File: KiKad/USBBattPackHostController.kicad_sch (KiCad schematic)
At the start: 21 parts, among them SW301 Reset, U305 MIC5201-3.3YS, U306 MIC5209-3.3YS, U307 MCP601-xOT, U401 STM32L422KBTx

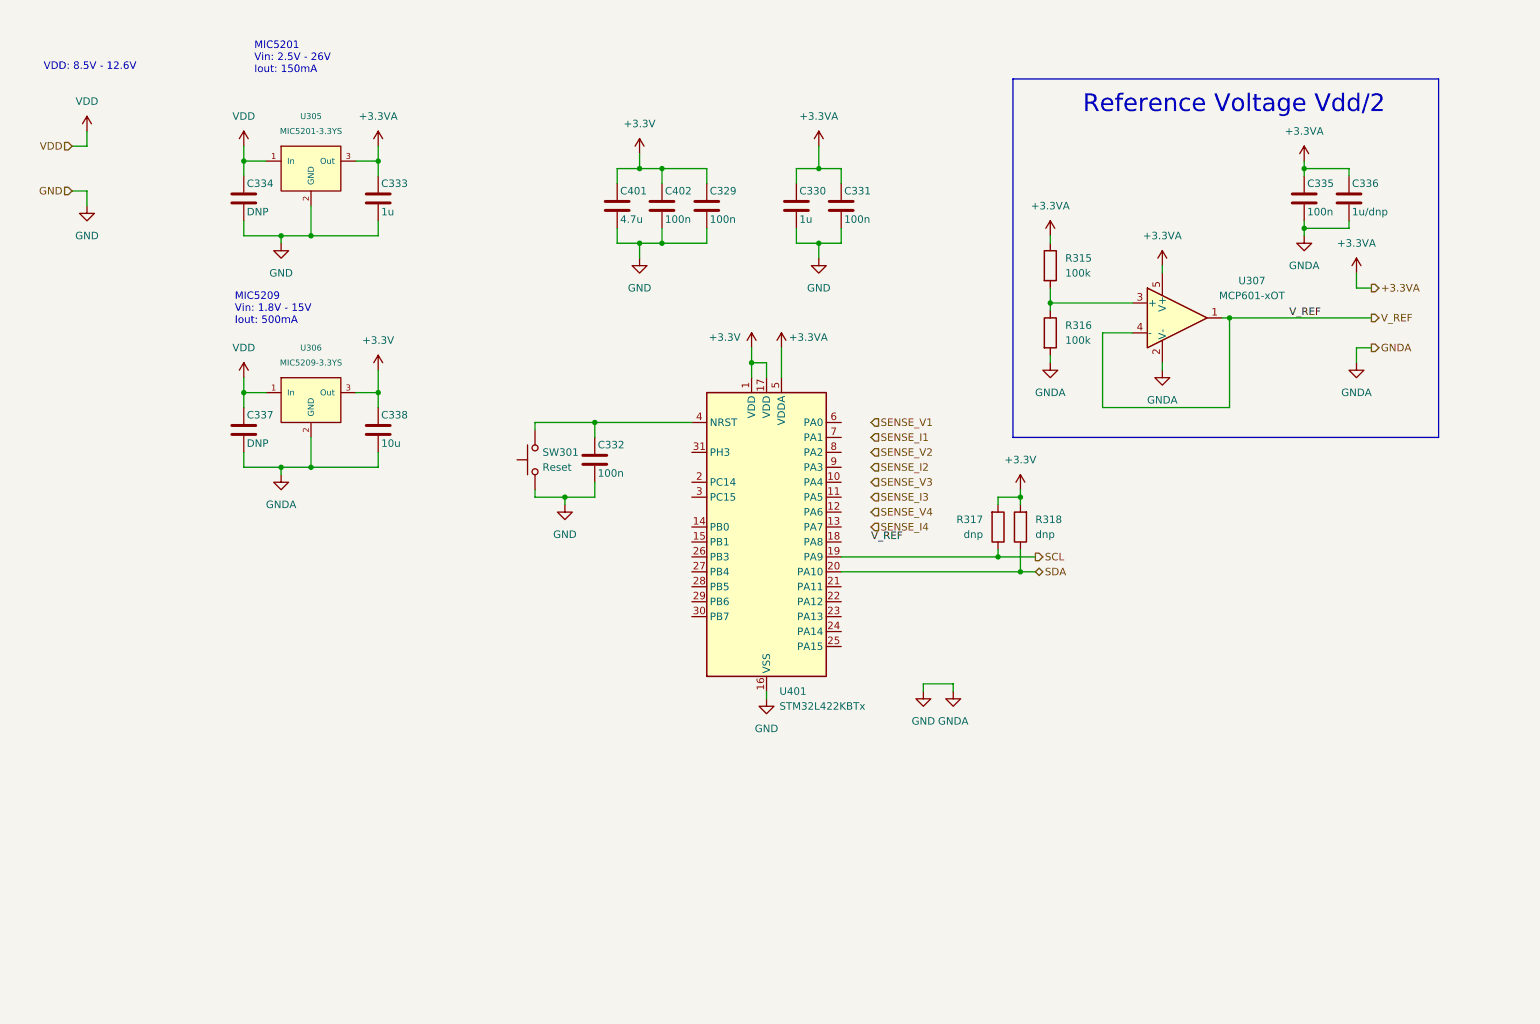
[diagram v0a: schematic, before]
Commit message: some work
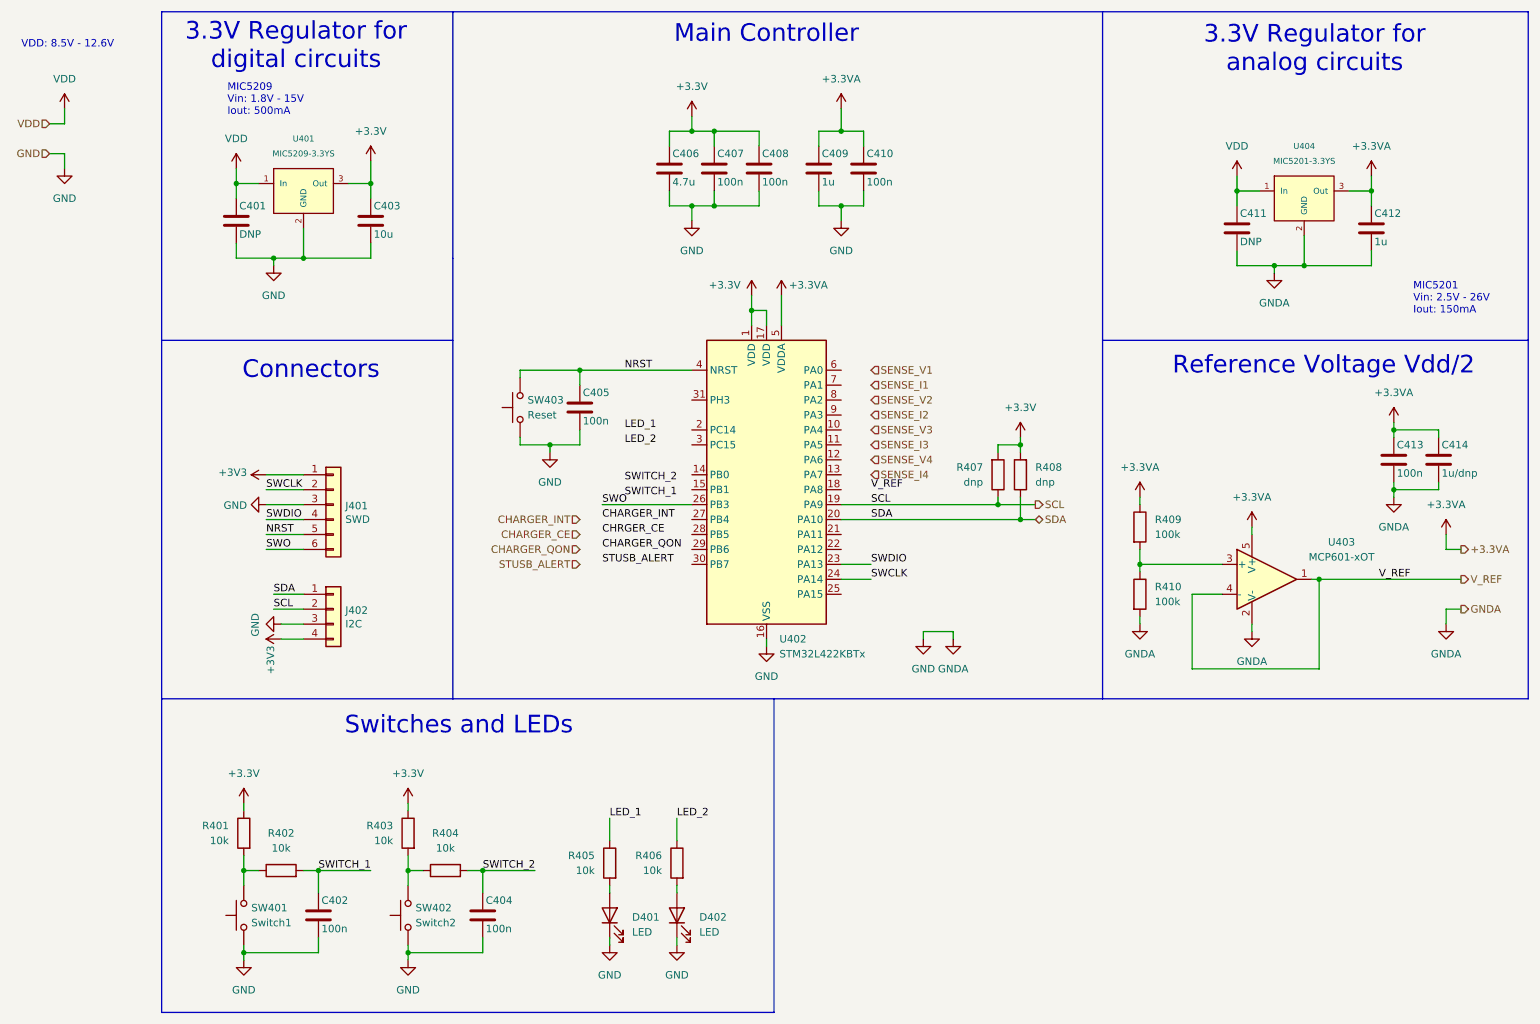
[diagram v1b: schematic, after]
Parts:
- added C402, C404: 100n, symbol Device:C
- added D401, D402: LED, symbol Device:LED
- added J401: SWD, Connector_JST:JST_PH_S6B-PH-SM4-TB_1x06-1MP_P2.00mm_Horizontal, symbol Connector_Generic:Conn_01x06
- added J402: I2C, JPConnectors:PinSocket_1x04_P2.54mm_Horizontal_SMD, symbol Connector_Generic:Conn_01x04
- added R401, R402, R403, R404, R405, R406: 10k, symbol Device:R
- added SW401: Switch1, symbol Switch:SW_Push
- added SW402: Switch2, symbol Switch:SW_Push
- renumbered C337 to C401, C338 to C403, C332 to C405, C401 to C406, C402 to C407, C329 to C408, C330 to C409, C331 to C410, C334 to C411, C333 to C412, C335 to C413, C336 to C414, R317 to R407, R318 to R408, R315 to R409, R316 to R410, SW301 to SW403, U306 to U401, U401 to U402, U307 to U403, U305 to U404
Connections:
- net +3.3V: now also R401.1, R403.1
- net GND: now also C402.2, C404.2, D401.1 (K), D402.1 (K), J401.3 (Pin_3), J402.3 (Pin_3), SW401.1, SW402.1
- net SCL: now also J402.2 (Pin_2)
- net SDA: now also J402.1 (Pin_1)
- net NRST: now reaches C405.1, SW403.2, U402.4 (NRST)
- net NRST: now also J401.5 (Pin_5)
- net SWDIO: now reaches U402.23 (PA13)
- net SWDIO: now also J401.4 (Pin_4)
- net SWCLK: now reaches U402.24 (PA14)
- net SWCLK: now also J401.2 (Pin_2)
- net SWO: now reaches U402.26 (PB3)
- net SWO: now also J401.6 (Pin_6)
- new net: R403.2, R404.1, SW402.2
- new net: R401.2, R402.1, SW401.2
- new net: D401.2 (A), R405.2
- new net: D402.2 (A), R406.2
- new net +3V3: J401.1 (Pin_1), J402.4 (Pin_4)
- new net LED_1: R405.1
- new net LED_2: R406.1
- new net SWITCH_1: C402.1, R402.2
- new net SWITCH_2: C404.1, R404.2
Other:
- note added: "3.3V Regulator for analog circuits"
- note added: "3.3V Regulator for digital circuits"
- note added: "Connectors"
- note added: "Main Controller"
- note added: "Switches and LEDs"
- moved on the sheet: C401, C403, C405, C406, C407, C408, C409, C410, C411, C412, C413, C414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
